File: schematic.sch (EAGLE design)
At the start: 27 parts, among them U1 EK-TM4C123GXL, U2 MCP23017-E/SP, U3 MCP23017-E/SP, U4 MCP23017-E/SP, U5 MCP23017-E/SP

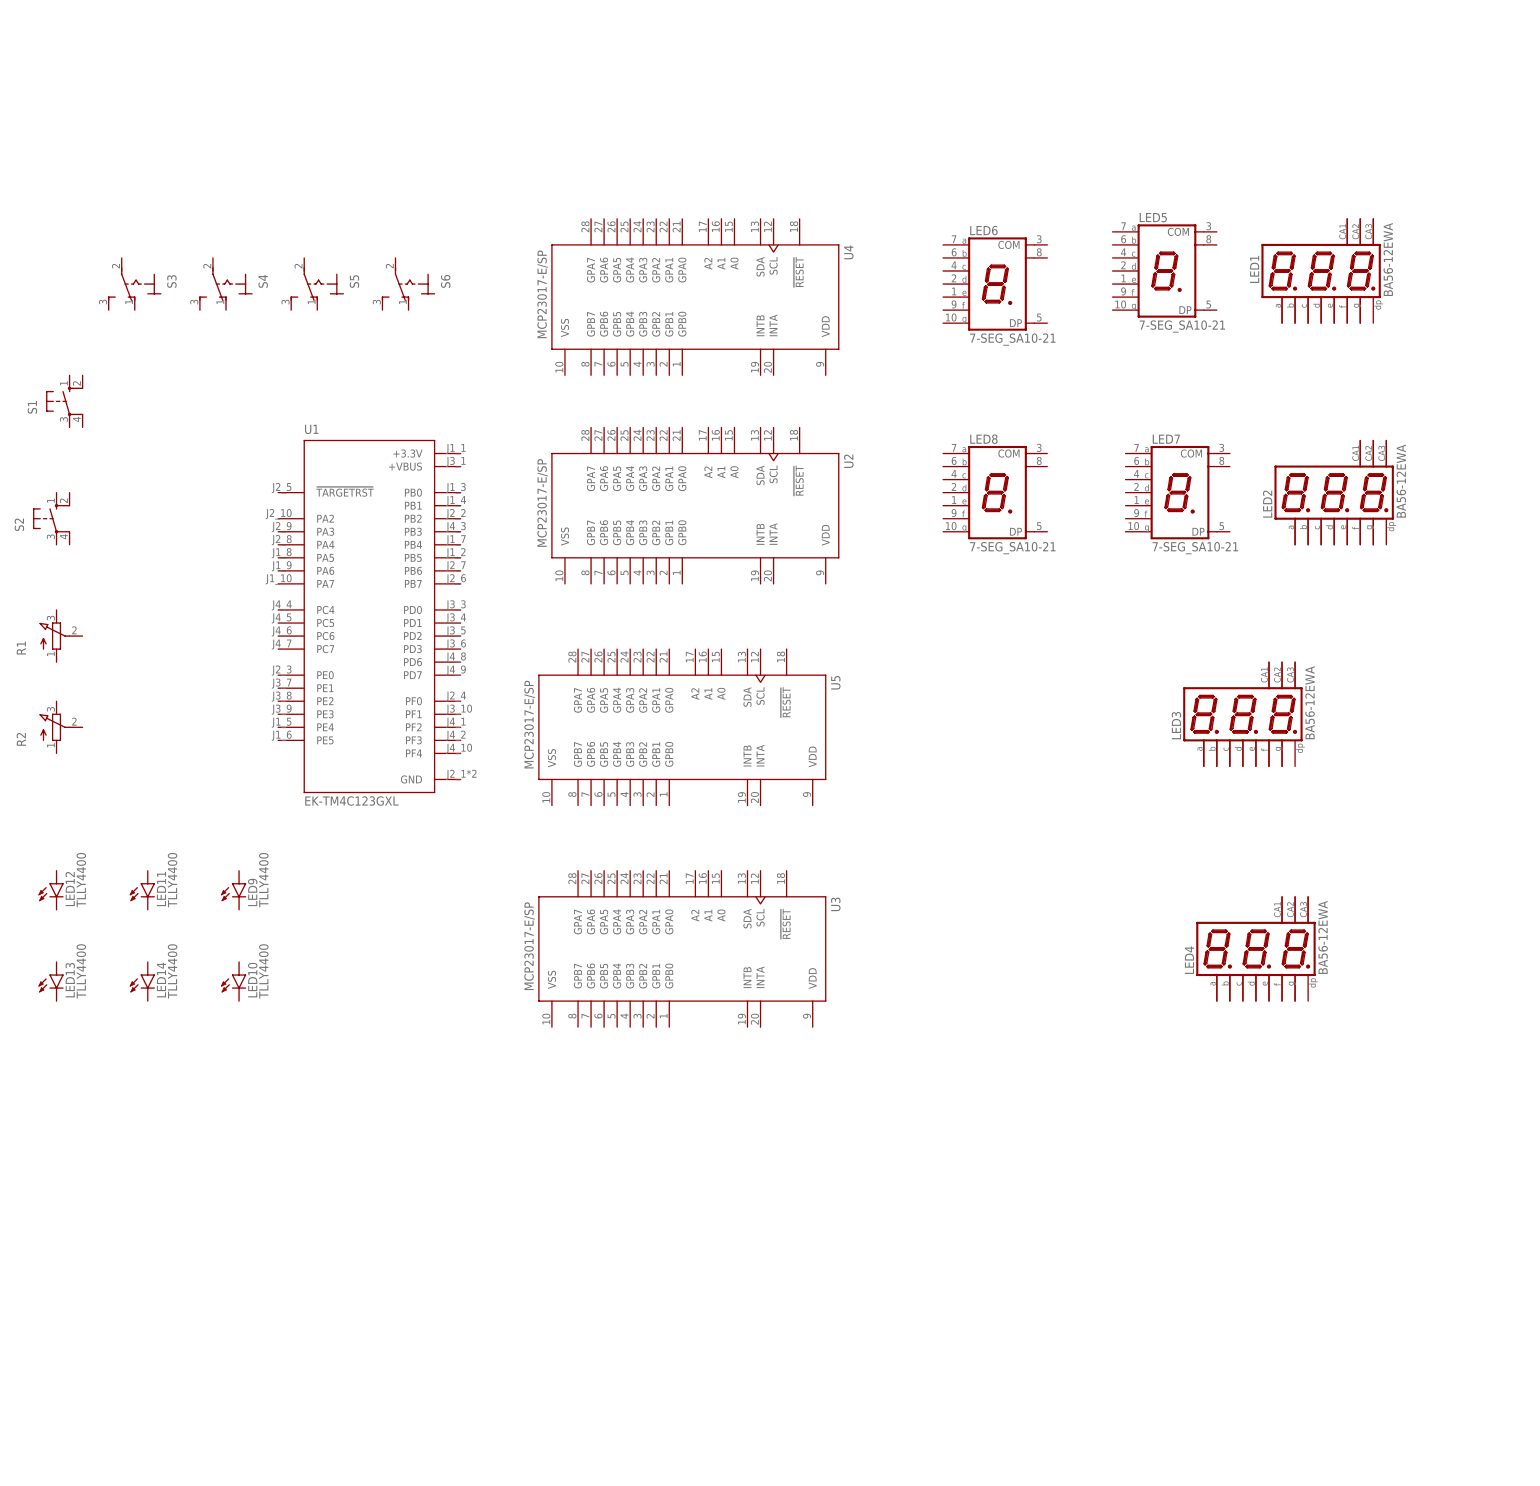
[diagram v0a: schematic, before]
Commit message: Update schematic.sch
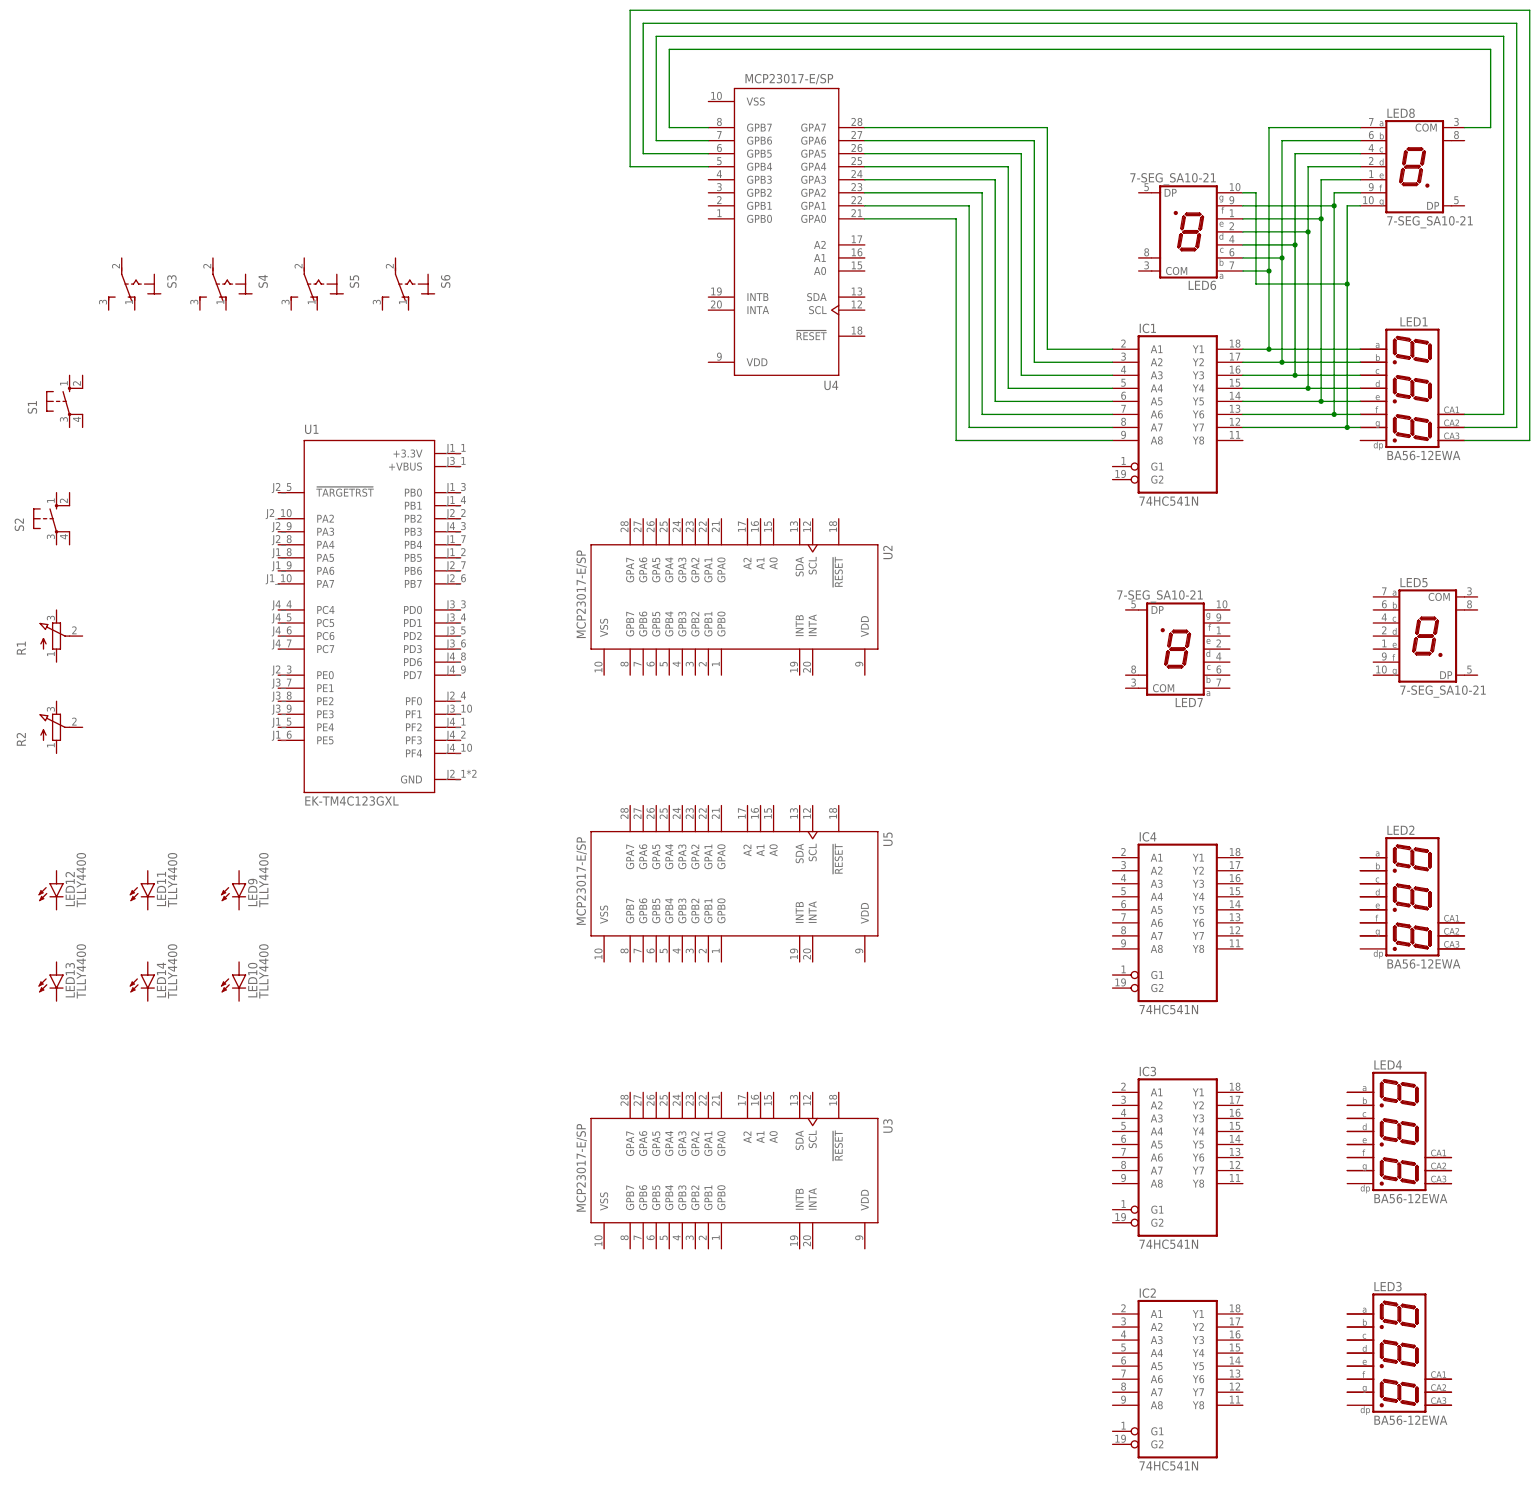
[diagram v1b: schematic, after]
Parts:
- added IC1, IC2, IC3, IC4: 74HC541N, 74xx-eu:74HC541N
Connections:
- new net N$1: IC1A.A8, U4.GPA0
- new net N$10: IC1A.A6, U4.GPA2
- new net N$11: IC1A.A5, U4.GPA3
- new net N$12: IC1A.A4, U4.GPA4
- new net N$13: IC1A.A3, U4.GPA5
- new net N$14: IC1A.A2, U4.GPA6
- new net N$15: IC1A.A1, U4.GPA7
- new net N$16: LED8.COM@1, U4.GPB7
- new net N$17: LED1.CA@1, U4.GPB6
- new net N$18: LED1.CA@2, U4.GPB5
- new net N$19: LED1.CA@3, U4.GPB4
- new net N$2: IC1A.Y2, LED1.B, LED6.B, LED8.B
- new net N$3: IC1A.Y3, LED1.C, LED6.C, LED8.C
- new net N$4: IC1A.Y4, LED1.D, LED6.D, LED8.D
- new net N$5: IC1A.Y5, LED1.E, LED6.E, LED8.E
- new net N$6: IC1A.Y6, LED1.F, LED6.F, LED8.F
- new net N$7: IC1A.Y7, LED1.G, LED6.G, LED8.G
- new net N$8: IC1A.Y1, LED1.A, LED6.A, LED8.A
- new net N$9: IC1A.A7, U4.GPA1
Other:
- moved on the sheet: LED1, LED2, LED3, LED4, LED5, LED6, LED7, LED8, U2, U3, U4, U5
